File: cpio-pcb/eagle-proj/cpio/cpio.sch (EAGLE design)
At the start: 67 parts

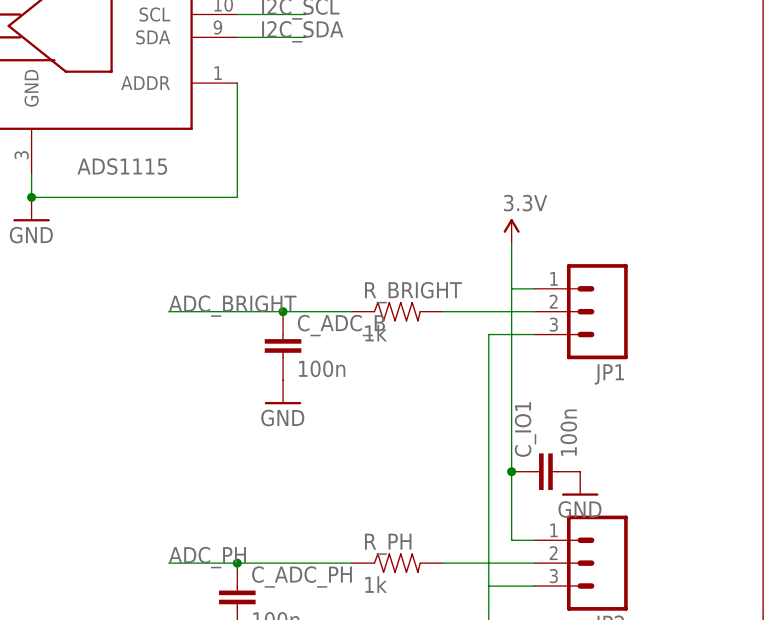
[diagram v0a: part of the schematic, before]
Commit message: schematic revs...
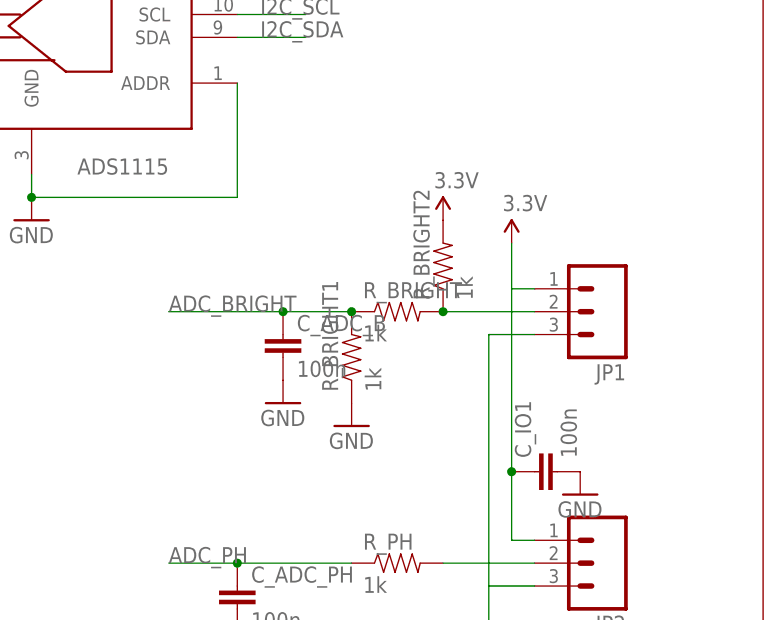
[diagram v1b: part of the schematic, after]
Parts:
- added R_BRIGHT1, R_BRIGHT2: 1k, SparkFun-Passives:RESISTOR0805-RES
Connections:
- net 3.3V: now also R_BRIGHT2.2
- net ADC_BRIGHT: now also R_BRIGHT1.2
- net GND: now also R_BRIGHT1.1
- net N$35: now also R_BRIGHT2.1
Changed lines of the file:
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@@
 <part name="LED1" library="led" deviceset="LED" device="SML0805"/>
 <part name="LED2" library="led" deviceset="LED" device="SML0805"/>
+<part name="R_BRIGHT1" library="SparkFun-Passives" deviceset="RESISTOR" device="0805-RES" value="1k"/>
+<part name="R_BRIGHT2" library="SparkFun-Passives" deviceset="RESISTOR" device="0805-RES" value="1k"/>
+<part name="SUPPLY12" library="SparkFun-Aesthetics" deviceset="3.3V" device=""/>
+<part name="GND10" library="supply1" deviceset="GND" device=""/>
 </parts>
 <sheets>
@@
 <instance part="LED1" gate="G$1" x="38.1" y="-66.04"/>
 <instance part="LED2" gate="G$1" x="264.16" y="-226.06"/>
+<instance part="R_BRIGHT1" gate="G$1" x="426.72" y="-208.28" rot="R90"/>
+<instance part="R_BRIGHT2" gate="G$1" x="436.88" y="-198.12" rot="R90"/>
+<instance part="SUPPLY12" gate="G$1" x="436.88" y="-193.04"/>
+<instance part="GND10" gate="1" x="426.72" y="-215.9"/>
 </instances>
 <busses>
@@
 <junction x="119.38" y="-147.32"/>
 </segment>
+<segment>
+<pinref part="R_BRIGHT1" gate="G$1" pin="1"/>
+<pinref part="GND10" gate="1" pin="GND"/>
+</segment>
 </net>
 <net name="GPIO17" class="0">
@@
 <pinref part="JP2" gate="G$1" pin="1"/>
 </segment>
+<segment>
+<pinref part="R_BRIGHT2" gate="G$1" pin="2"/>
+<pinref part="SUPPLY12" gate="G$1" pin="3.3V"/>
+</segment>
 </net>
 <net name="N$15" class="0">
@@
 <wire x1="447.04" y1="-203.2" x2="436.88" y2="-203.2" width="0.1524" layer="91"/>
 <pinref part="JP1" gate="G$1" pin="2"/>
+<pinref part="R_BRIGHT2" gate="G$1" pin="1"/>
+<junction x="436.88" y="-203.2"/>
 </segment>
 </net>
@@
 <wire x1="419.1" y1="-203.2" x2="406.4" y2="-203.2" width="0.1524" layer="91"/>
 <junction x="419.1" y="-203.2"/>
-</segment>
-<segment>
+<pinref part="R_BRIGHT1" gate="G$1" pin="2"/>
+<junction x="426.72" y="-203.2"/>
+</segment>
+<segment>
